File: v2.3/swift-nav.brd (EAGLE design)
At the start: 53 x 53 mm, 157 parts, among them J1 SMA_EDGE, J6 ZX62-B-5PA, Q1 IRLML6401, U1 6SLX9FTG256, U10 MAX2769, U12 PT7M8206B33TA5EX, U13 M25PX80, U2 LTC3407A_DFN, U3 STM32-M-64-LQFP, U4 7Q-16.368MBG-T, U5 SMA_PATCH_SMDGND, U6 93LC56BT-I/OT, U7 FT232HQ, U8 B4050, U9 XC2401, X3 FPGA DEBUG, X4 NX5032GA-12M, X5 CONN_5-2

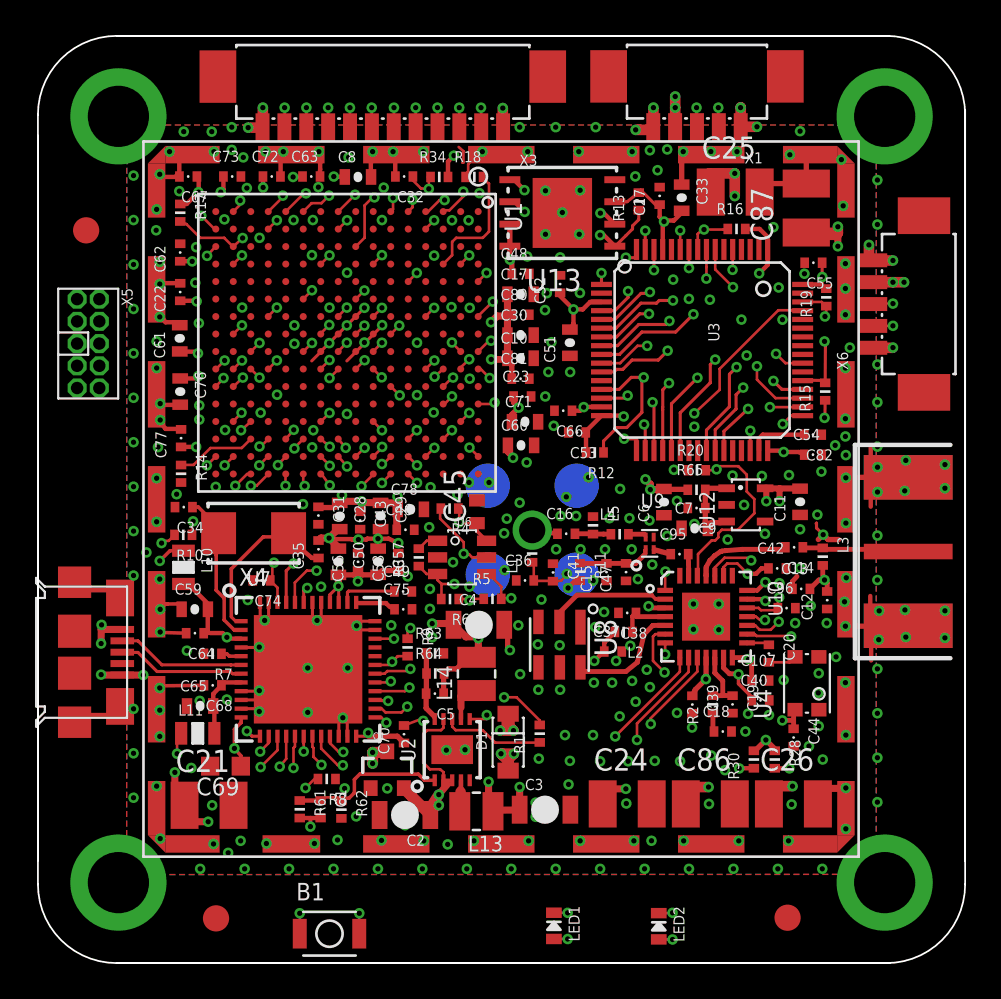
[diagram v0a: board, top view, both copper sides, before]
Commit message: v2.3 as sent out for production
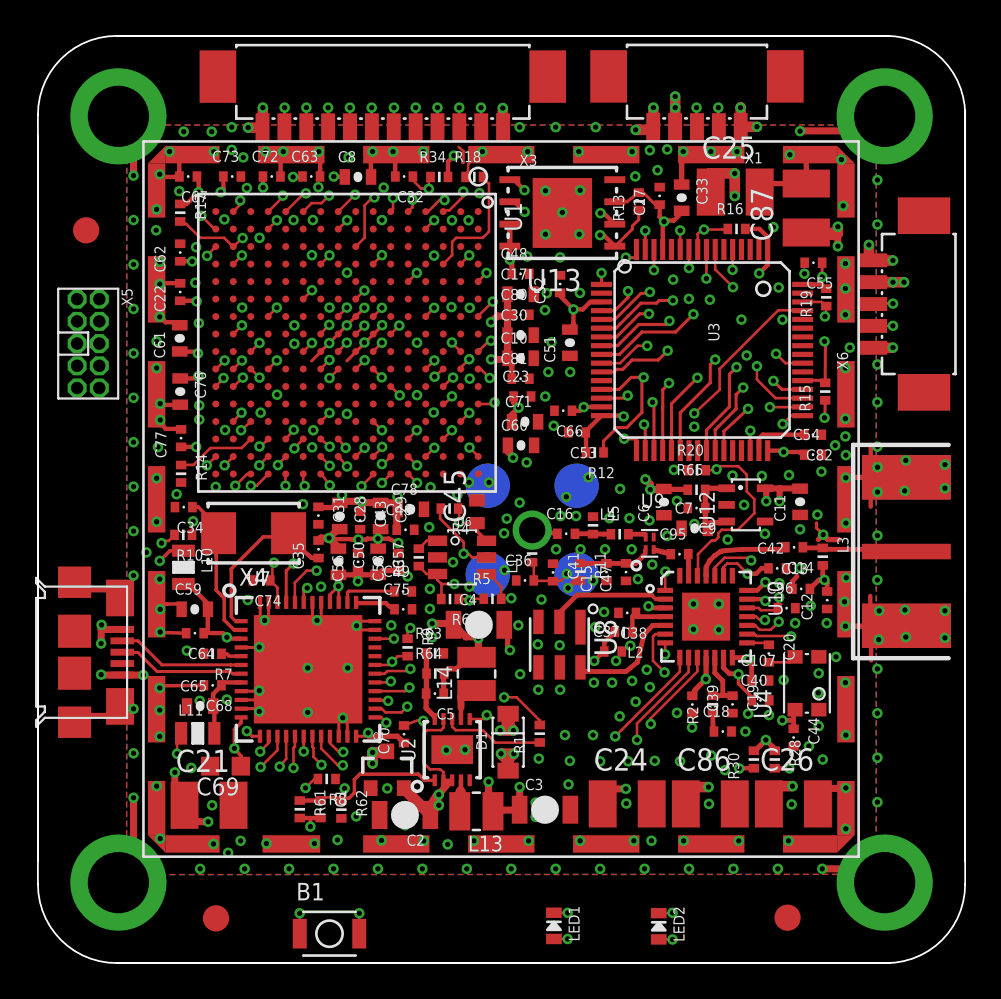
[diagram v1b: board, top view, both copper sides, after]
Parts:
- moved J1 0.10 mm to (55.6, 26.9)
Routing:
- net GND: track 122.0 -> 153.6 mm
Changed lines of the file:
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@@
 <setting verticaltext="up"/>
 </settings>
-<grid distance="0.3" unitdist="mil" unit="mil" style="lines" multiple="1" display="yes" altdistance="0.25" altunitdist="mil" altunit="mil"/>
+<grid distance="1" unitdist="mil" unit="mil" style="lines" multiple="1" display="yes" altdistance="0.25" altunitdist="mil" altunit="mil"/>
 <layers>
 <layer number="1" name="Top" color="4" fill="1" visible="no" active="yes"/>
@@
 <layer number="14" name="Route14" color="1" fill="6" visible="no" active="yes"/>
 <layer number="15" name="Route15" color="4" fill="6" visible="no" active="yes"/>
-<layer number="16" name="Bottom" color="1" fill="1" visible="no" active="yes"/>
+<layer number="16" name="Bottom" color="1" fill="1" visible="yes" active="yes"/>
 <layer number="17" name="Pads" color="2" fill="1" visible="yes" active="yes"/>
-<layer number="18" name="Vias" color="2" fill="1" visible="no" active="yes"/>
-<layer number="19" name="Unrouted" color="6" fill="1" visible="no" active="yes"/>
+<layer number="18" name="Vias" color="2" fill="1" visible="yes" active="yes"/>
+<layer number="19" name="Unrouted" color="6" fill="1" visible="yes" active="yes"/>
 <layer number="20" name="Dimension" color="15" fill="1" visible="yes" active="yes"/>
 <layer number="21" name="tPlace" color="7" fill="1" visible="no" active="yes"/>
-<layer number="22" name="bPlace" color="7" fill="1" visible="no" active="yes"/>
+<layer number="22" name="bPlace" color="7" fill="1" visible="yes" active="yes"/>
 <layer number="23" name="tOrigins" color="15" fill="1" visible="no" active="yes"/>
-<layer number="24" name="bOrigins" color="15" fill="1" visible="no" active="yes"/>
+<layer number="24" name="bOrigins" color="15" fill="1" visible="yes" active="yes"/>
 <layer number="25" name="tNames" color="7" fill="1" visible="no" active="yes"/>
 <layer number="26" name="bNames" color="7" fill="1" visible="no" active="yes"/>
@@
 <layer number="28" name="bValues" color="7" fill="1" visible="no" active="yes"/>
 <layer number="29" name="tStop" color="7" fill="3" visible="no" active="yes"/>
-<layer number="30" name="bStop" color="7" fill="6" visible="no" active="yes"/>
+<layer number="30" name="bStop" color="7" fill="6" visible="yes" active="yes"/>
 <layer number="31" name="tCream" color="7" fill="4" visible="no" active="yes"/>
 <layer number="32" name="bCream" color="7" fill="5" visible="no" active="yes"/>
@@
 <param name="mdViaViaSameLayer" value="8mil"/>
 <param name="mnLayersViaInSmd" value="2"/>
-<param name="mdCopperDimension" value="25mil"/>
+<param name="mdCopperDimension" value="30mil"/>
 <param name="mdDrill" value="8mil"/>
 <param name="mdSmdStop" value="0mil"/>
@@
 <element name="B1" library="jobygnss" package="B3U-1000P" value="B3U-1000P" x="20.066" y="5.08"/>
 <element name="U5" library="joby_robotics" package="SMA_PATCH_SMDGND" value="SMA_PATCH_SMDGND" x="29.9" y="29.9" rot="MR270"/>
-<element name="J1" library="swift-nav" package="SMA_EDGE" value="SMA_EDGE" x="55.686959375" y="26.924" smashed="yes" rot="R270"/>
+<element name="J1" library="swift-nav" package="SMA_EDGE" value="SMA_EDGE" x="55.585359375" y="26.924" smashed="yes" rot="R270"/>
 <element name="C2" library="pel_dipol_comp" package="1206-CAP" value="10uF" x="24.3796" y="11.8646" rot="R180"/>
 <element name="C3" library="pel_dipol_comp" package="1206-CAP" value="10uF" x="32.385" y="12.1666"/>
@@
 <wire x1="7.0104" y1="19.8882" x2="8.8392" y2="19.8882" width="0.4064" layer="14"/>
 <via x="25.7654" y="28.3139" extent="1-16" drill="0.3"/>
-<wire x1="49.3268" y1="49.3268" x2="51.8" y2="51.8" width="0" layer="19" extent="1-1"/>
-<wire x1="53.009" y1="22.0354" x2="53.146959375" y2="22.6822" width="0" layer="19" extent="16-16"/>
-<wire x1="52.945" y1="30.3944" x2="53.146959375" y2="31.1658" width="0" layer="19" extent="16-16"/>
-<wire x1="52.959" y1="23.5854" x2="53.146959375" y2="22.6822" width="0" layer="19" extent="16-16"/>
-<wire x1="53.009" y1="32.1334" x2="53.146959375" y2="31.1658" width="0" layer="19" extent="16-16"/>
-<wire x1="55.245" y1="30.5444" x2="53.146959375" y2="31.1658" width="0" layer="19" extent="16-16"/>
-<wire x1="55.245" y1="31.8944" x2="55.245" y2="30.5444" width="0" layer="19" extent="1-1"/>
-<wire x1="55.245" y1="21.9894" x2="53.146959375" y2="22.6822" width="0" layer="19" extent="16-16"/>
-<wire x1="55.245" y1="23.5394" x2="55.245" y2="21.9894" width="0" layer="19" extent="1-1"/>
-<wire x1="8" y1="8" x2="10.3886" y2="10.5156" width="0" layer="19" extent="1-1"/>
-<wire x1="8" y1="51.8" x2="8.8646" y2="48.4124" width="0" layer="19" extent="1-1"/>
-<wire x1="51.8" y1="8" x2="48.2346" y2="8.7884" width="0" layer="19" extent="1-1"/>
+<wire x1="48.2346" y1="8.7884" x2="51.8" y2="8.7884" width="0.4064" layer="1"/>
+<wire x1="51.8" y1="8.7884" x2="51.8" y2="8" width="0.4064" layer="1"/>
+<wire x1="8" y1="8" x2="8.79348125" y2="8" width="0.4064" layer="1"/>
+<wire x1="8.79348125" y1="8" x2="8.79348125" y2="8.900159375" width="0.4064" layer="1"/>
+<wire x1="8.79348125" y1="8.900159375" x2="8.8646" y2="8.900159375" width="0.4064" layer="1"/>
+<wire x1="8.8646" y1="8.900159375" x2="8.8646" y2="12.8524" width="0.4064" layer="1"/>
+<wire x1="8" y1="51.8" x2="8.8646" y2="51.8" width="0.4064" layer="1"/>
+<wire x1="8.8646" y1="51.8" x2="8.8646" y2="48.4124" width="0.4064" layer="1"/>
+<wire x1="51.8" y1="51.8" x2="50.6349" y2="51.8" width="0.4064" layer="1"/>
+<wire x1="50.6349" y1="51.8" x2="50.6349" y2="50.97018125" width="0.4064" layer="1"/>
+<wire x1="50.6349" y1="50.97018125" x2="46.9646" y2="50.97018125" width="0.4064" layer="1"/>
+<wire x1="46.9646" y1="50.97018125" x2="46.9646" y2="50.9524" width="0.4064" layer="1"/>
+<wire x1="52.959" y1="23.5854" x2="53.009" y2="23.5854" width="0.4064" layer="1"/>
+<wire x1="53.009" y1="23.5854" x2="53.009" y2="22.0354" width="0.4064" layer="1"/>
+<wire x1="53.009" y1="22.0354" x2="55.245" y2="22.0354" width="0.4064" layer="1"/>
+<wire x1="55.245" y1="22.0354" x2="55.245" y2="21.9894" width="0.4064" layer="1"/>
+<wire x1="55.245" y1="22.0354" x2="55.245" y2="23.5394" width="0.4064" layer="1"/>
+<wire x1="53.009" y1="22.0354" x2="53.146959375" y2="22.0354" width="0.4064" layer="1"/>
+<wire x1="53.146959375" y1="22.0354" x2="53.045359375" y2="22.6822" width="0.4064" layer="1"/>
+<wire x1="55.245" y1="31.8944" x2="55.245" y2="30.5444" width="0.4064" layer="1"/>
+<wire x1="55.245" y1="30.5444" x2="53.146959375" y2="30.5444" width="0.4064" layer="1"/>
+<wire x1="52.945" y1="30.5444" x2="52.945" y2="30.3944" width="0.4064" layer="1"/>
+<wire x1="52.945" y1="30.5444" x2="53.146959375" y2="30.5444" width="0.4064" layer="1"/>
+<wire x1="53.146959375" y1="30.5444" x2="53.045359375" y2="31.1658" width="0.4064" layer="1"/>
+<wire x1="53.045359375" y1="31.1658" x2="53.009" y2="31.1658" width="0.4064" layer="1"/>
+<wire x1="53.009" y1="31.1658" x2="53.009" y2="32.1334" width="0.4064" layer="1"/>
 </signal>
 <signal name="N$3">
@@
 <wire x1="47.196759375" y1="27.08514375" x2="47.122959375" y2="27.167675" width="0.2286" layer="1"/>
 <contactref element="L3" pad="P$1"/>
-<wire x1="53.146959375" y1="26.924" x2="50.8762" y2="26.924" width="0.2794" layer="1"/>
+<wire x1="53.045359375" y1="26.924" x2="50.8762" y2="26.924" width="0.2794" layer="1"/>
 <wire x1="50.8762" y1="26.924" x2="50.7492" y2="27.051" width="0.2794" layer="1"/>
 <wire x1="50.7492" y1="27.051" x2="48.3409" y2="27.051" width="0.2794" layer="1"/>
